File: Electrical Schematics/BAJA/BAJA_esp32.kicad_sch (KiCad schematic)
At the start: 9 parts

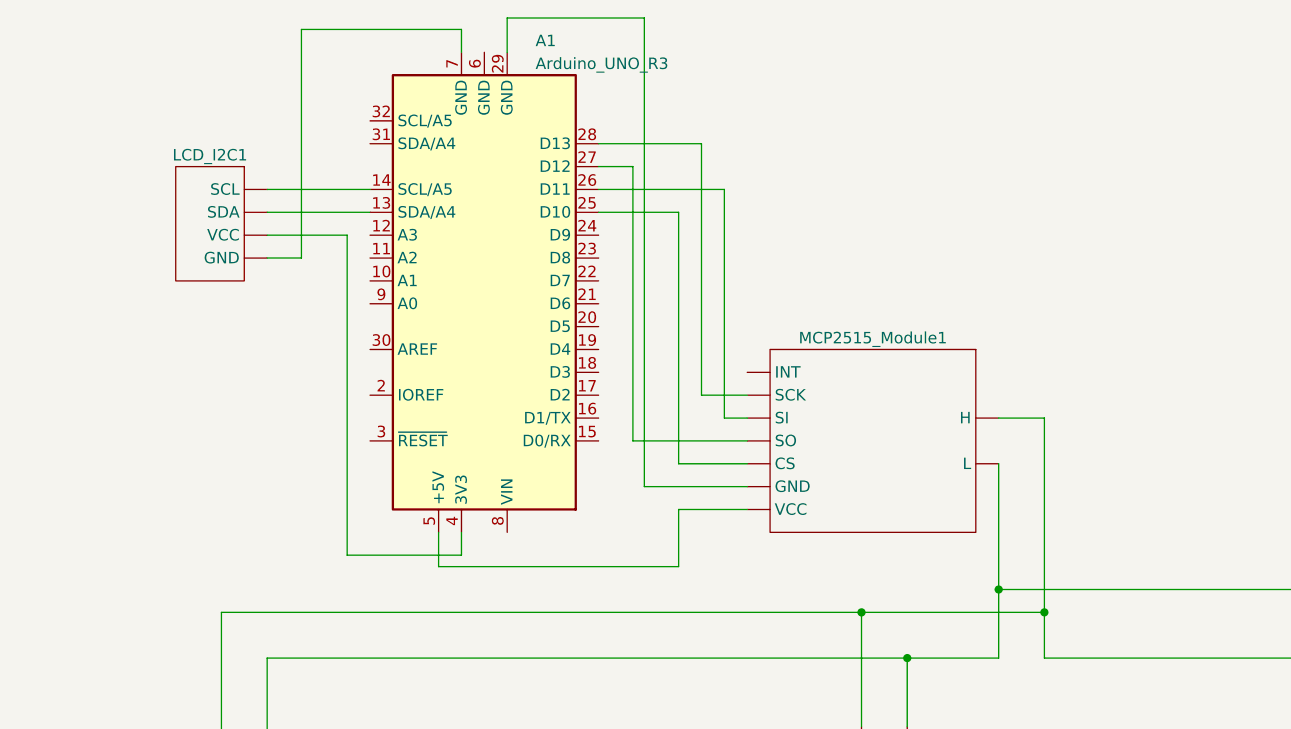
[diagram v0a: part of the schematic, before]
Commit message: new file management
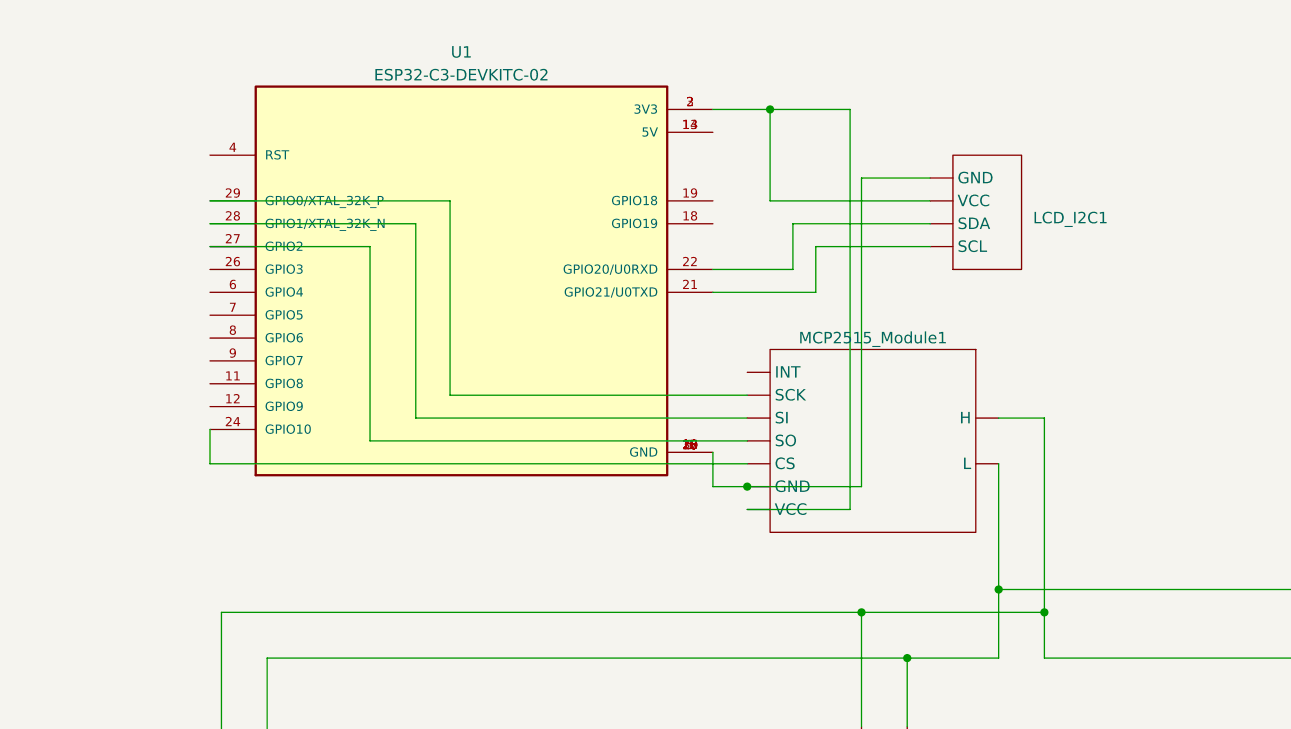
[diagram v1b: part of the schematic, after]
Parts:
- removed A1: Arduino_UNO_R3, Module:Arduino_UNO_R3, symbol MCU_Module:Arduino_UNO_R3
- added U1: ESP32-C3-DEVKITC-02, XCVR_ESP32-C3-DEVKITC-02, symbol ESP32-C3-DEVKITC-02:ESP32-C3-DEVKITC-02
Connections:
- net at MCP2515_Module2. (VCC): now also MCP2515_Module1. (VCC), MCP2515_Module3. (VCC), MCP2515_Module4. (VCC)
- net at MCP2515_Module4. (VCC): now also A2.4 (GND)
- net at MCP2515_Module3. (VCC): now also A3.4 (GND)
- net at LCD_I2C1. (VCC): now also U1.22 (GPIO20/U0RXD)
- new net: MCP2515_Module1. (VCC), MCP2515_Module2. (VCC), MCP2515_Module3. (VCC), MCP2515_Module4. (VCC)
- new net: LCD_I2C1. (VCC), MCP2515_Module1. (VCC), U1.1 (GND), U1.10 (GND), U1.15 (GND), U1.16 (GND), U1.17 (GND), U1.20 (GND), U1.23 (GND), U1.25 (GND), U1.30 (GND), U1.5 (GND)
- new net: U1.13 (5V), U1.14 (5V)
- new net: LCD_I2C1. (VCC), MCP2515_Module1. (VCC), U1.2 (3V3), U1.3 (3V3)
- new net: LCD_I2C1. (VCC), U1.21 (GPIO21/U0TXD)
- new net: MCP2515_Module1. (VCC), U1.24 (GPIO10)
- new net: MCP2515_Module1. (VCC), U1.27 (GPIO2)
- new net: MCP2515_Module1. (VCC), U1.28 (GPIO1/XTAL_32K_N)
- new net: MCP2515_Module1. (VCC), U1.29 (GPIO0/XTAL_32K_P)
- now unconnected: MCP2515_Module1. (VCC), MCP2515_Module1. (VCC), MCP2515_Module1. (VCC), MCP2515_Module1. (VCC), MCP2515_Module1. (VCC), MCP2515_Module1. (VCC), MCP2515_Module1. (VCC)
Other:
- moved on the sheet: LCD_I2C1

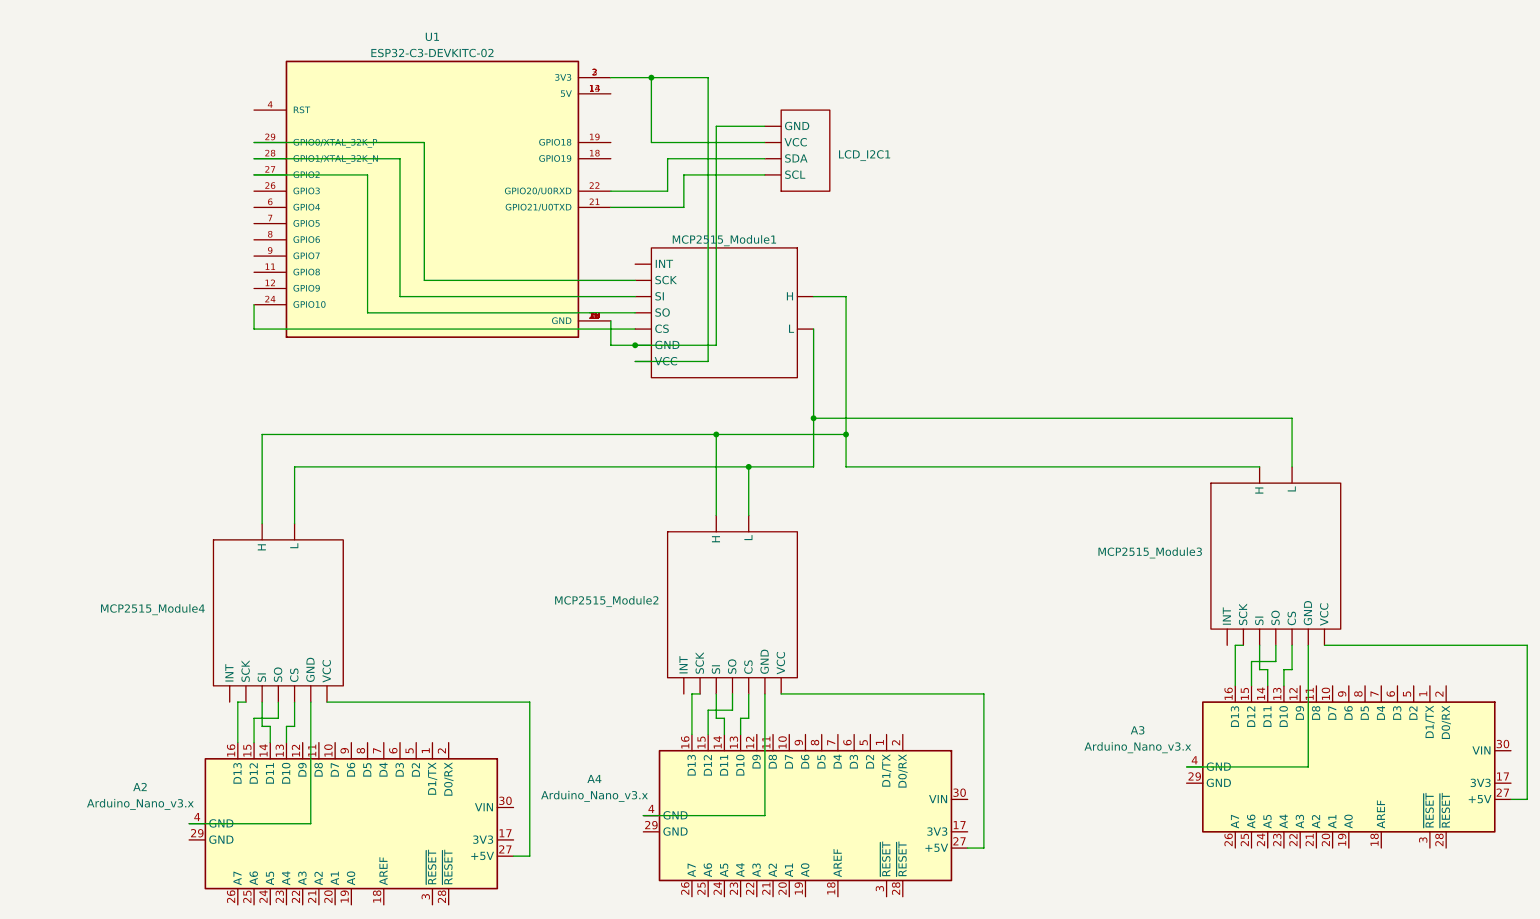
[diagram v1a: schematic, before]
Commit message: updated esp32 schematics
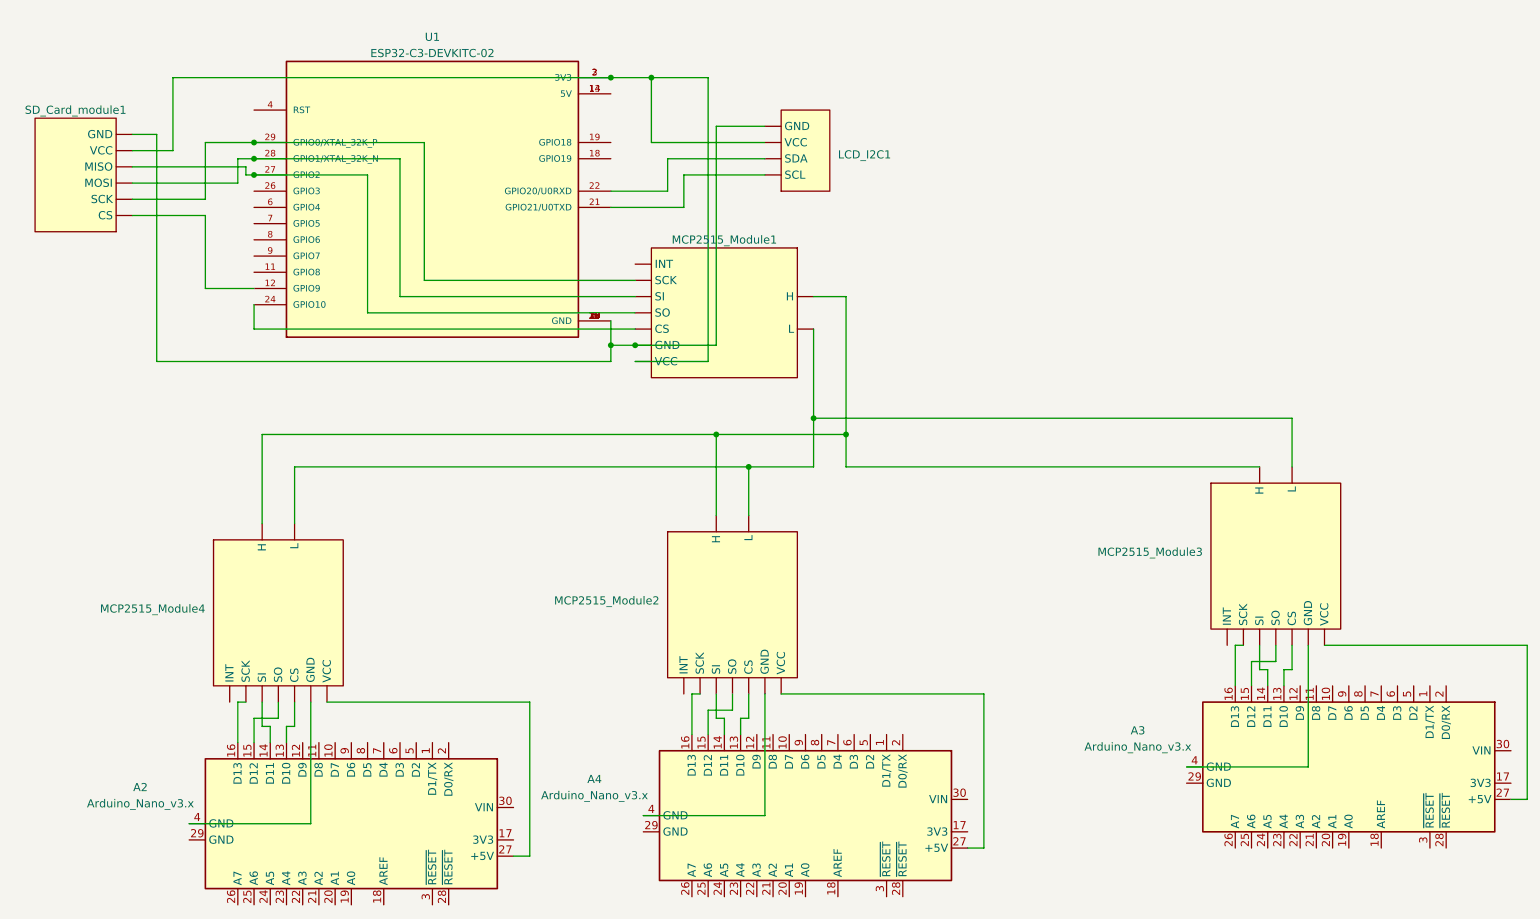
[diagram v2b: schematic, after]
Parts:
- added SD_Card_module1: ~, symbol BAJA:SD_Card_Module
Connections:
- net at MCP2515_Module2. (VCC): now also MCP2515_Module1. (VCC), MCP2515_Module3. (VCC), MCP2515_Module4. (VCC)
- net at MCP2515_Module4. (VCC): now also A2.4 (GND)
- net at MCP2515_Module3. (VCC): now also A3.4 (GND)
- net at LCD_I2C1. (VCC), MCP2515_Module1. (VCC), U1.1 (GND)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: now also SD_Card_module1. (VCC)
- net at U1.12 (GPIO9): now also SD_Card_module1. (VCC)
- net at LCD_I2C1. (VCC), MCP2515_Module1. (VCC), U1.2 (3V3)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: now also SD_Card_module1. (VCC)
- net at MCP2515_Module1. (VCC), U1.27 (GPIO2): now also SD_Card_module1. (VCC)
- net at MCP2515_Module1. (VCC), U1.28 (GPIO1/XTAL_32K_N): now also SD_Card_module1. (VCC)
- net at MCP2515_Module1. (VCC), U1.29 (GPIO0/XTAL_32K_P): now also SD_Card_module1. (VCC)
- new net: MCP2515_Module1. (VCC), MCP2515_Module2. (VCC), MCP2515_Module3. (VCC), MCP2515_Module4. (VCC)
- now unconnected: MCP2515_Module1. (VCC), MCP2515_Module1. (VCC)
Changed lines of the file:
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@@
   (junction (at 119.38 71.12) (diameter 0) (color 0 0 0 0)
   )
+  (junction (at 115.57 71.12) (diameter 0) (color 0 0 0 0)
+  )
+  (junction (at 115.57 29.21) (diameter 0) (color 0 0 0 0)
+  )
+  (junction (at 59.69 41.91) (diameter 0) (color 0 0 0 0)
+  )
   (junction (at 121.92 29.21) (diameter 0) (color 0 0 0 0)
   )
@@
   (junction (at 137.16 90.17) (diameter 0) (color 0 0 0 0)
   )
+  (junction (at 59.69 39.37) (diameter 0) (color 0 0 0 0)
+  )
   (junction (at 152.4 85.09) (diameter 0) (color 0 0 0 0)
   )
+  (junction (at 59.69 44.45) (diameter 0) (color 0 0 0 0)
+  )
   (wire (pts (xy 102.87 127) (xy 71.12 127))
     (stroke (width 0) (type default))
@@
     (stroke (width 0) (type default))
   )
+  (wire (pts (xy 44.45 73.66) (xy 115.57 73.66))
+    (stroke (width 0) (type default))
+  )
+  (wire (pts (xy 52.07 62.23) (xy 59.69 62.23))
+    (stroke (width 0) (type default))
+  )
   (wire (pts (xy 152.4 85.09) (xy 152.4 63.5))
     (stroke (width 0) (type default))
@@
     (stroke (width 0) (type default))
   )
+  (wire (pts (xy 40.64 40.64) (xy 46.99 40.64))
+    (stroke (width 0) (type default))
+  )
+  (wire (pts (xy 52.07 48.26) (xy 52.07 39.37))
+    (stroke (width 0) (type default))
+  )
   (wire (pts (xy 66.04 90.17) (xy 66.04 99.06))
     (stroke (width 0) (type default))
   )
+  (wire (pts (xy 58.42 43.18) (xy 58.42 44.45))
+    (stroke (width 0) (type default))
+  )
   (wire (pts (xy 218.44 124.46) (xy 218.44 121.92))
     (stroke (width 0) (type default))
@@
     (stroke (width 0) (type default))
   )
+  (wire (pts (xy 44.45 38.1) (xy 44.45 73.66))
+    (stroke (width 0) (type default))
+  )
   (wire (pts (xy 121.92 29.21) (xy 115.57 29.21))
     (stroke (width 0) (type default))
@@
     (stroke (width 0) (type default))
   )
+  (wire (pts (xy 57.15 45.72) (xy 57.15 41.91))
+    (stroke (width 0) (type default))
+  )
+  (wire (pts (xy 40.64 43.18) (xy 58.42 43.18))
+    (stroke (width 0) (type default))
+  )
   (wire (pts (xy 147.32 90.17) (xy 147.32 82.55))
     (stroke (width 0) (type default))
@@
     (stroke (width 0) (type default))
   )
+  (wire (pts (xy 115.57 73.66) (xy 115.57 71.12))
+    (stroke (width 0) (type default))
+  )
+  (wire (pts (xy 40.64 38.1) (xy 44.45 38.1))
+    (stroke (width 0) (type default))
+  )
   (wire (pts (xy 173.99 125.73) (xy 142.24 125.73))
     (stroke (width 0) (type default))
@@
     (stroke (width 0) (type default))
   )
+  (wire (pts (xy 46.99 29.21) (xy 115.57 29.21))
+    (stroke (width 0) (type default))
+  )
+  (wire (pts (xy 52.07 39.37) (xy 59.69 39.37))
+    (stroke (width 0) (type default))
+  )
   (wire (pts (xy 139.7 144.78) (xy 120.65 144.78))
     (stroke (width 0) (type default))
@@
     (stroke (width 0) (type default))
   )
+  (wire (pts (xy 46.99 40.64) (xy 46.99 29.21))
+    (stroke (width 0) (type default))
+  )
   (wire (pts (xy 119.38 60.96) (xy 86.36 60.96))
     (stroke (width 0) (type default))
@@
     (stroke (width 0) (type default))
   )
+  (wire (pts (xy 40.64 50.8) (xy 52.07 50.8))
+    (stroke (width 0) (type default))
+  )
   (wire (pts (xy 135.89 132.08) (xy 135.89 129.54))
     (stroke (width 0) (type default))
@@
     (stroke (width 0) (type default))
   )
+  (wire (pts (xy 58.42 44.45) (xy 59.69 44.45))
+    (stroke (width 0) (type default))
+  )
   (wire (pts (xy 77.47 44.45) (xy 59.69 44.45))
     (stroke (width 0) (type default))
   )
+  (wire (pts (xy 52.07 50.8) (xy 52.07 62.23))
+    (stroke (width 0) (type default))
+  )
   (wire (pts (xy 130.81 128.27) (xy 134.62 128.27))
     (stroke (width 0) (type default))
@@
     (stroke (width 0) (type default))
   )
+  (wire (pts (xy 57.15 41.91) (xy 59.69 41.91))
+    (stroke (width 0) (type default))
+  )
+  (wire (pts (xy 217.17 90.17) (xy 152.4 90.17))
+    (stroke (width 0) (type default))
+  )
+  (wire (pts (xy 130.81 73.66) (xy 130.81 29.21))
+    (stroke (width 0) (type default))
+  )
+  (wire (pts (xy 119.38 63.5) (xy 82.55 63.5))
+    (stroke (width 0) (type default))
+  )
+  (wire (pts (xy 40.64 48.26) (xy 52.07 48.26))
+    (stroke (width 0) (type default))
+  )
+  (wire (pts (xy 256.54 142.24) (xy 259.08 142.24))
+    (stroke (width 0) (type default))
+  )
   (wire (pts (xy 59.69 41.91) (xy 82.55 41.91))
     (stroke (width 0) (type default))
   )
-  (wire (pts (xy 217.17 90.17) (xy 152.4 90.17))
-    (stroke (width 0) (type default))
-  )
-  (wire (pts (xy 130.81 73.66) (xy 130.81 29.21))
-    (stroke (width 0) (type default))
-  )
-  (wire (pts (xy 119.38 63.5) (xy 82.55 63.5))
-    (stroke (width 0) (type default))
-  )
-  (wire (pts (xy 256.54 142.24) (xy 259.08 142.24))
-    (stroke (width 0) (type default))
-  )
   (wire (pts (xy 173.99 149.86) (xy 173.99 125.73))
     (stroke (width 0) (type default))
@@
     (stroke (width 0) (type default))
   )
+  (wire (pts (xy 40.64 45.72) (xy 57.15 45.72))
+    (stroke (width 0) (type default))
+  )
   (wire (pts (xy 82.55 63.5) (xy 82.55 41.91))
     (stroke (width 0) (type default))
@@
     (stroke (width 0) (type default))
   )
-  (symbol (lib_name "MCP2515_Module_3") (lib_id "BAJA:MCP2515_Module") (at 134.62 102.87 0) (unit 1)
+  (symbol (lib_name "MCP2515_Module_1") (lib_id "BAJA:MCP2515_Module") (at 134.62 102.87 0) (unit 1)
     (in_bom yes) (on_board yes) (dnp no) (fields_autoplaced)
     (property "Reference" "MCP2515_Module2" (at 123.19 111.125 0)
@@
     )
   )
-  (symbol (lib_name "MCP2515_Module_3") (lib_id "BAJA:MCP2515_Module") (at 63.5 104.14 0) (unit 1)
+  (symbol (lib_id "BAJA:MCP2515_Module") (at 63.5 104.14 0) (unit 1)
     (in_bom yes) (on_board yes) (dnp no) (fields_autoplaced)
     (property "Reference" "MCP2515_Module4" (at 52.07 112.395 0)
@@
         )
       )
+    )
+  )
+  (symbol (lib_id "BAJA:SD_Card_Module") (at 30.48 45.72 180) (unit 1)
+    (in_bom yes) (on_board yes) (dnp no) (fields_autoplaced)
+    (property "Reference" "SD_Card_module1" (at 31.75 34.29 0)
+      (effects (font (size 1.27 1.27)))
+    )
+    (property "Value" "~" (at 30.48 45.72 0)
+      (effects (font (size 1.27 1.27)))
+    )
+    (property "Footprint" "" (at 30.48 45.72 0)
+      (effects (font (size 1.27 1.27)) hide)
+    )
+    (property "Datasheet" "" (at 30.48 45.72 0)
+      (effects (font (size 1.27 1.27)) hide)
+    )
+    (pin "")
+    (pin "")
+    (pin "")
+    (pin "")
+    (pin "")
+    (pin "")
+    (instances
+      (project "BAJA_esp32"
+        (path "/47f460ff-5de8-4d8f-925a-72af6b9a6795"
+          (reference "SD_Card_module1") (unit 1)
+        )
+      )
